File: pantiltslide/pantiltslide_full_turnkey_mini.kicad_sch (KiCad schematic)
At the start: 57 parts, among them J1 Conn_01x22_Socket, J17 Motor_Slide, J18 Motor_Pan, J19 Motor_Tilt, J2 Conn_01x22_Socket, J20 TCA9548A_Mux, J21 AS5600_Pan, J22 AS5600_Tilt, J23 OLED, J24 TCA9548A_Mux, J26 Limit_Min, J27 Limit_Max, J28 Motor_Aux, J29 Enc_Slide, J30 Enc_Pan, J31 Enc_Tilt, J32 Enc_Aux, J33 Btn_SetKeyframe, J34 Btn_ClearKeyframe, J35 Btn_PlayPause, J36 Btn_Reset, J37 5V_In, J38 24V_In, J41 Aux_Max, U1 tmc2209, U2 tmc2209, U3 tmc2209, U4 tmc2209

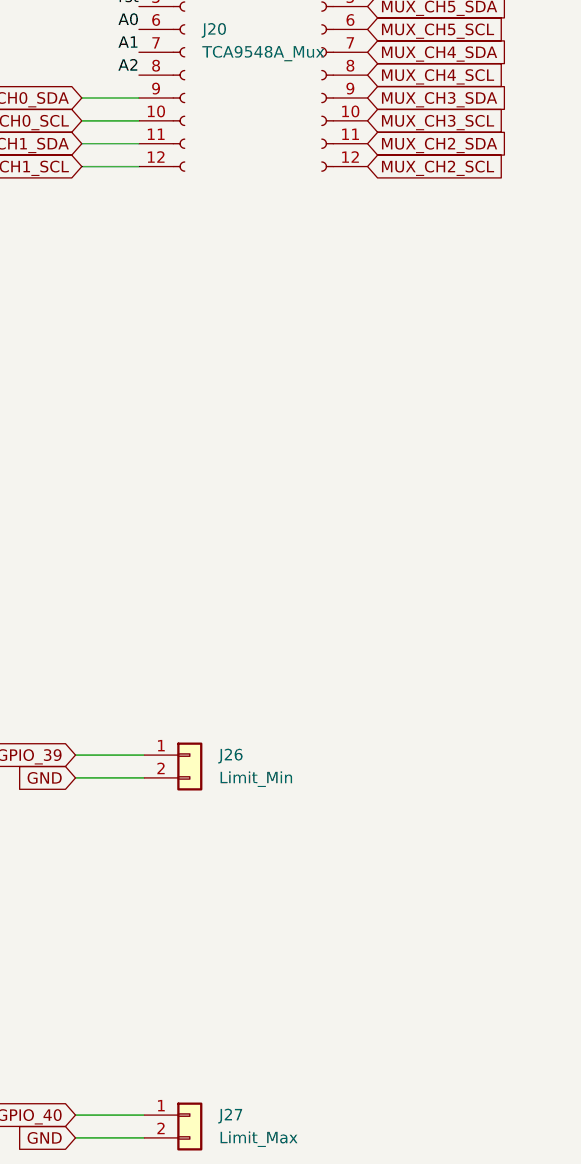
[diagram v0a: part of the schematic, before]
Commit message: updastes
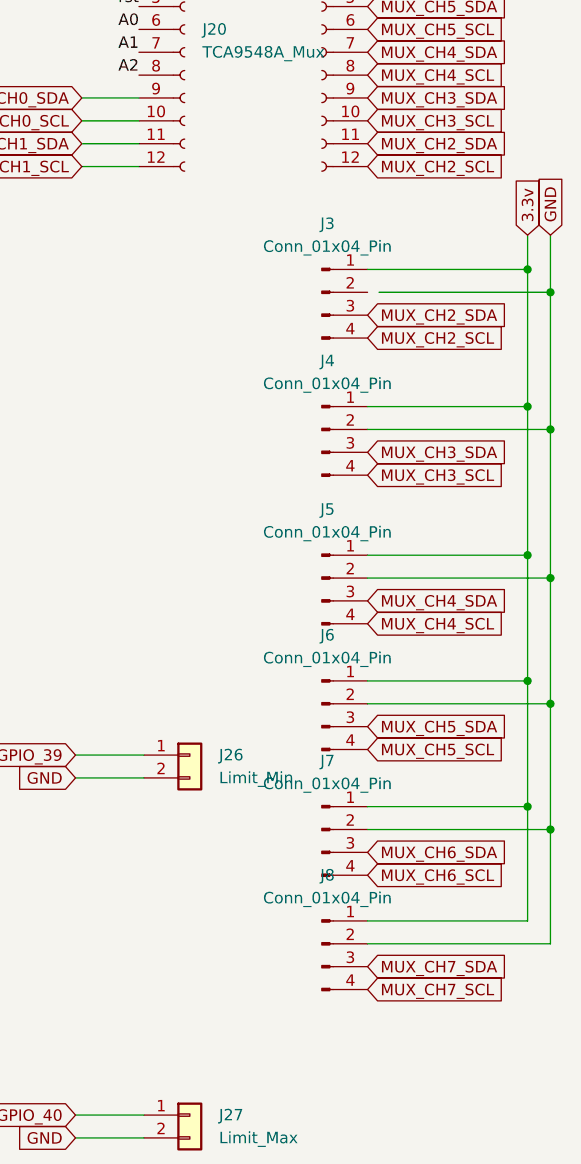
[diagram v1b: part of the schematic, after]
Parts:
- added J3, J4, J5, J6, J7, J8: Conn_01x04_Pin, symbol Connector:Conn_01x04_Pin
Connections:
- net +3.3V: now also J3.1 (Pin_1), J4.1 (Pin_1), J5.1 (Pin_1), J6.1 (Pin_1), J7.1 (Pin_1), J8.1 (Pin_1)
- net GND: now also J4.2 (Pin_2), J5.2 (Pin_2), J6.2 (Pin_2), J7.2 (Pin_2), J8.2 (Pin_2)
- net MUX_CH2_SCL: now also J3.4 (Pin_4)
- net MUX_CH2_SDA: now also J3.3 (Pin_3)
- net MUX_CH3_SCL: now also J4.4 (Pin_4)
- net MUX_CH3_SDA: now also J4.3 (Pin_3)
- net MUX_CH4_SCL: now also J5.4 (Pin_4)
- net MUX_CH4_SDA: now also J5.3 (Pin_3)
- net MUX_CH5_SCL: now also J6.4 (Pin_4)
- net MUX_CH5_SDA: now also J6.3 (Pin_3)
- net MUX_CH6_SCL: now also J7.4 (Pin_4)
- net MUX_CH6_SDA: now also J7.3 (Pin_3)
- net MUX_CH7_SCL: now also J8.4 (Pin_4)
- net MUX_CH7_SDA: now also J8.3 (Pin_3)
